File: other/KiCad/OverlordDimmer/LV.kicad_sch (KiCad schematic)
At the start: 99 parts, among them J3 Conn_01x12_Pin, U11 SN65HVD230

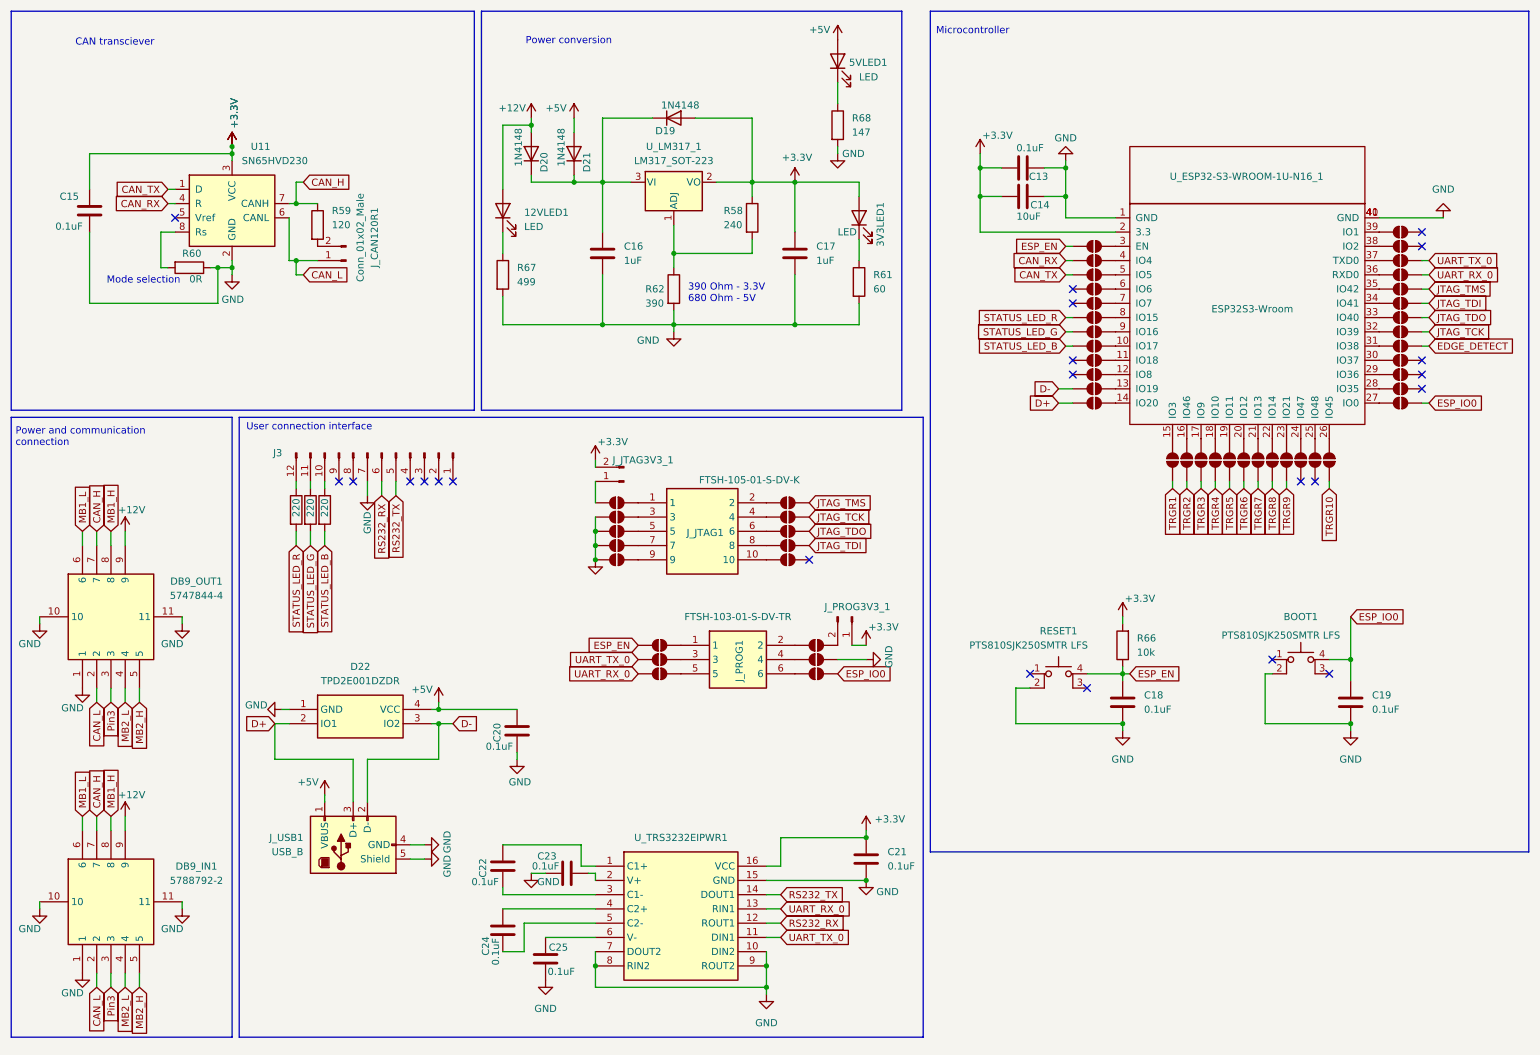
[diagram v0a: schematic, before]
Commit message: sent to production with fixes
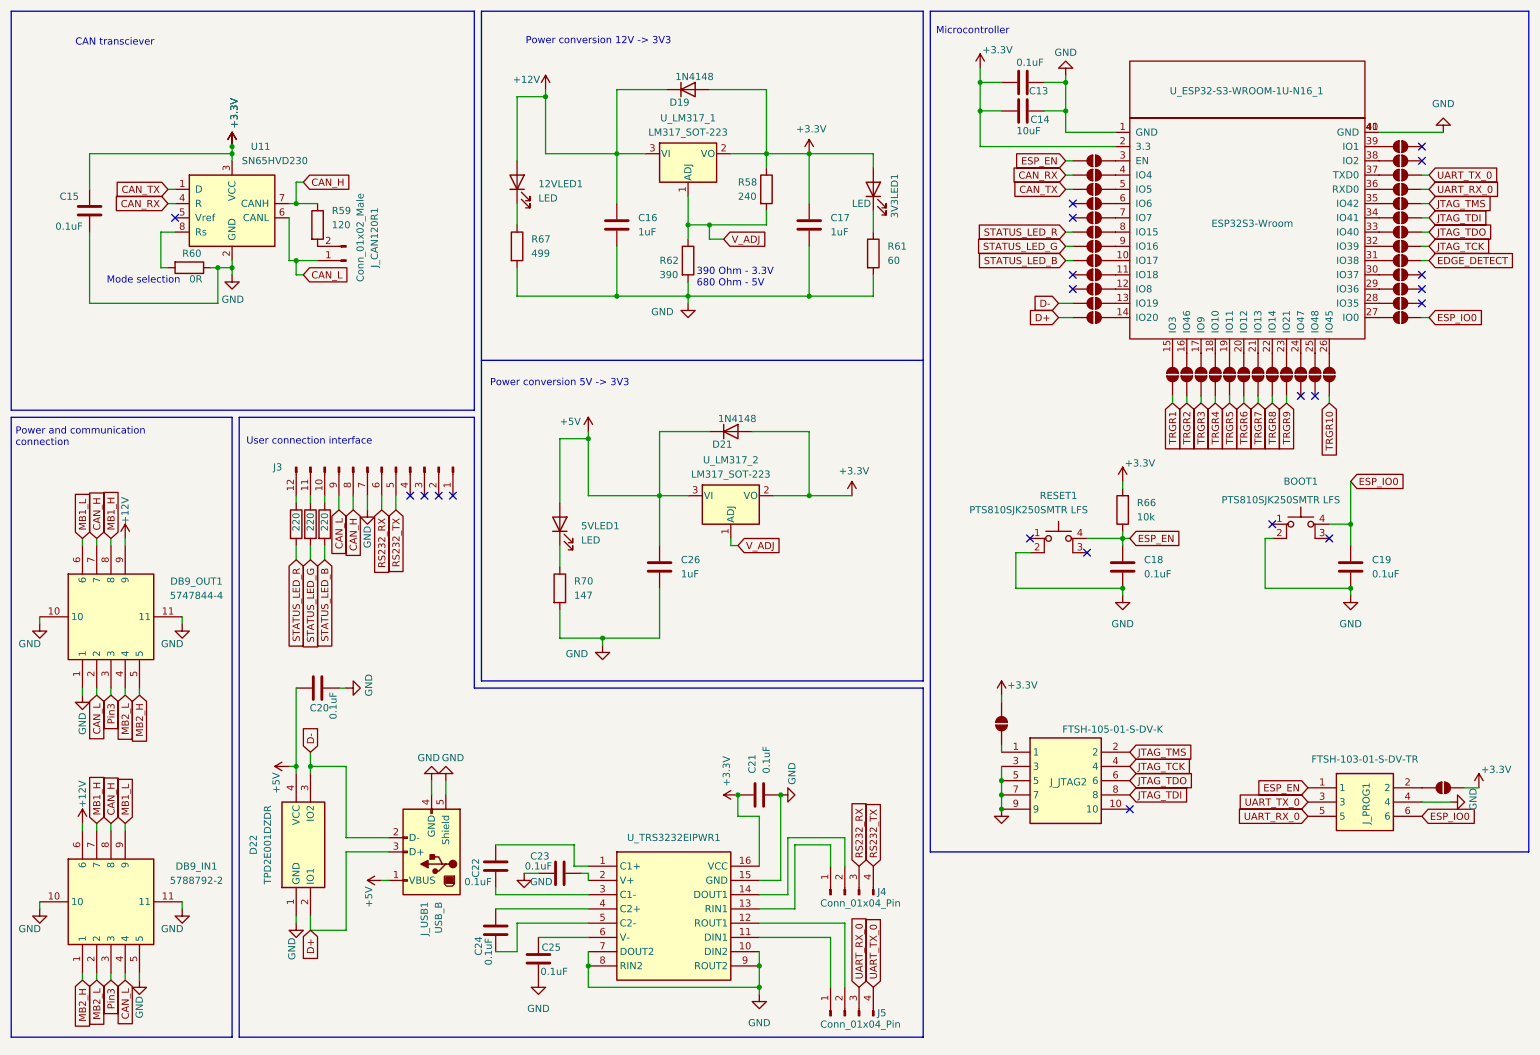
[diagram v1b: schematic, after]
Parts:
- removed D20: 1N4148, Diode_SMD:D_0805_2012Metric_Pad1.15x1.40mm_HandSolder, symbol Diode:1N4148
- removed JP38, JP39, JP40, JP42, JP43, JP44, JP45, JP46, JP47, JP48, JP50, JP51, JP52, JP53: SolderJumper_2_Open, Jumper:SolderJumper-2_P1.3mm_Open_RoundedPad1.0x1.5mm, symbol Jumper:SolderJumper_2_Open
- removed J_JTAG1: FTSH-105-01-S-DV-K, OverlordCommon:FTSH-105-XX-YYY-DV-K, symbol FTSH-105-01-S-DV-K:FTSH-105-01-S-DV-K
- removed J_JTAG3V3_1, J_PROG3V3_1: Conn_01x02_Pin, Connector_PinHeader_2.54mm:PinHeader_1x02_P2.54mm_Vertical, symbol Connector:Conn_01x02_Pin
- removed R68: 147, Resistor_SMD:R_0805_2012Metric_Pad1.20x1.40mm_HandSolder, symbol Device:R
- added C26: 1uF, Capacitor_SMD:C_0805_2012Metric_Pad1.18x1.45mm_HandSolder, symbol Device:C
- added J4, J5: Conn_01x04_Pin, OverlordCommon:Solder_select_2x2, symbol Connector:Conn_01x04_Pin
- added J_JTAG2: FTSH-105-01-S-DV-K, OverlordCommon:FTSH-105-XX-YYY-DV-K, symbol FTSH-105-01-S-DV-K:FTSH-105-01-S-DV-K
- added R70: 147, Resistor_SMD:R_0805_2012Metric_Pad1.20x1.40mm_HandSolder, symbol Device:R
- added U_LM317_2: LM317_SOT-223, Package_TO_SOT_SMD:SOT-223-3_TabPin2, symbol Regulator_Linear:LM317_SOT-223
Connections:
- net +12V: now also C16.1, D19.1 (K), DB9_IN1.6, U_LM317_1.3 (VI); no longer DB9_IN1.9
- net +3.3V: now also D21.2 (A), JP41.2 (B), JP49.2 (B), U_LM317_2.2 (VO)
- net +5V: now also D21.1 (K), C26.1, U_LM317_2.3 (VI); no longer D21.2 (A)
- net CAN_H: now also DB9_IN1.8, J3.8 (Pin_8); no longer DB9_IN1.7
- net CAN_L: now also DB9_IN1.4, J3.9 (Pin_9); no longer DB9_IN1.2
- net ESP_EN: now also J_PROG1.1
- net ESP_IO0: now also J_PROG1.6
- net GND: now also DB9_IN1.5, J_PROG1.4, C26.2, J_JTAG2.3, J_JTAG2.5, J_JTAG2.7, J_JTAG2.9, R70.2; no longer DB9_IN1.1
- net JTAG_TCK: now also J_JTAG2.4; no longer JP41.2 (B)
- net JTAG_TDI: now also J_JTAG2.8
- net JTAG_TDO: now also J_JTAG2.6
- net JTAG_TMS: now also J_JTAG2.2
- net MB1_H: now also DB9_IN1.7; no longer DB9_IN1.8
- net MB1_L: now also DB9_IN1.9; no longer DB9_IN1.6
- net MB2_H: now also DB9_IN1.1; no longer DB9_IN1.5
- net MB2_L: now also DB9_IN1.2; no longer DB9_IN1.4
- net RS232_RX: now also J4.3 (Pin_3); no longer U_TRS3232EIPWR1.12 (ROUT1)
- net RS232_TX: now also J4.4 (Pin_4); no longer U_TRS3232EIPWR1.14 (DOUT1)
- net UART_RX_0: now also J_PROG1.5, J5.3 (Pin_3); no longer U_TRS3232EIPWR1.13 (RIN1)
- net UART_TX_0: now also J_PROG1.3, J5.4 (Pin_4); no longer U_TRS3232EIPWR1.11 (DIN1)
- net V_ADJ: now reaches R58.2, R62.1, U_LM317_1.1 (ADJ)
- net V_ADJ: now also U_LM317_2.1 (ADJ)
- net at 5VLED1.1 (K): now also R70.1
- net at JP41.1 (A): now also J_JTAG2.1
- new net: J4.1 (Pin_1), U_TRS3232EIPWR1.13 (RIN1)
- new net: J4.2 (Pin_2), U_TRS3232EIPWR1.14 (DOUT1)
- new net: J5.1 (Pin_1), U_TRS3232EIPWR1.11 (DIN1)
- new net: J5.2 (Pin_2), U_TRS3232EIPWR1.12 (ROUT1)
- no-connect marks 23 -> 21
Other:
- note added: "Power conversion 12V -> 3V3"
- note added: "Power conversion 5V -> 3V3"
- note removed: "Power conversion"
- moved on the sheet: 12VLED1, 3V3LED1, BOOT1, C13, C14, C16, C17, C18, C19, C20, C21, C22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
